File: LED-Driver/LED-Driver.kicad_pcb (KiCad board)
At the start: 2 copper layers, 40.6 x 22.9 mm, 27 parts, among them P1 CONN_02X04, P2 CONN_02X04, P3 CONN_01X05, P4 CONN_01X02, P5 CONN_01X09, P6 CONN_01X09, U1 IS31FL3732

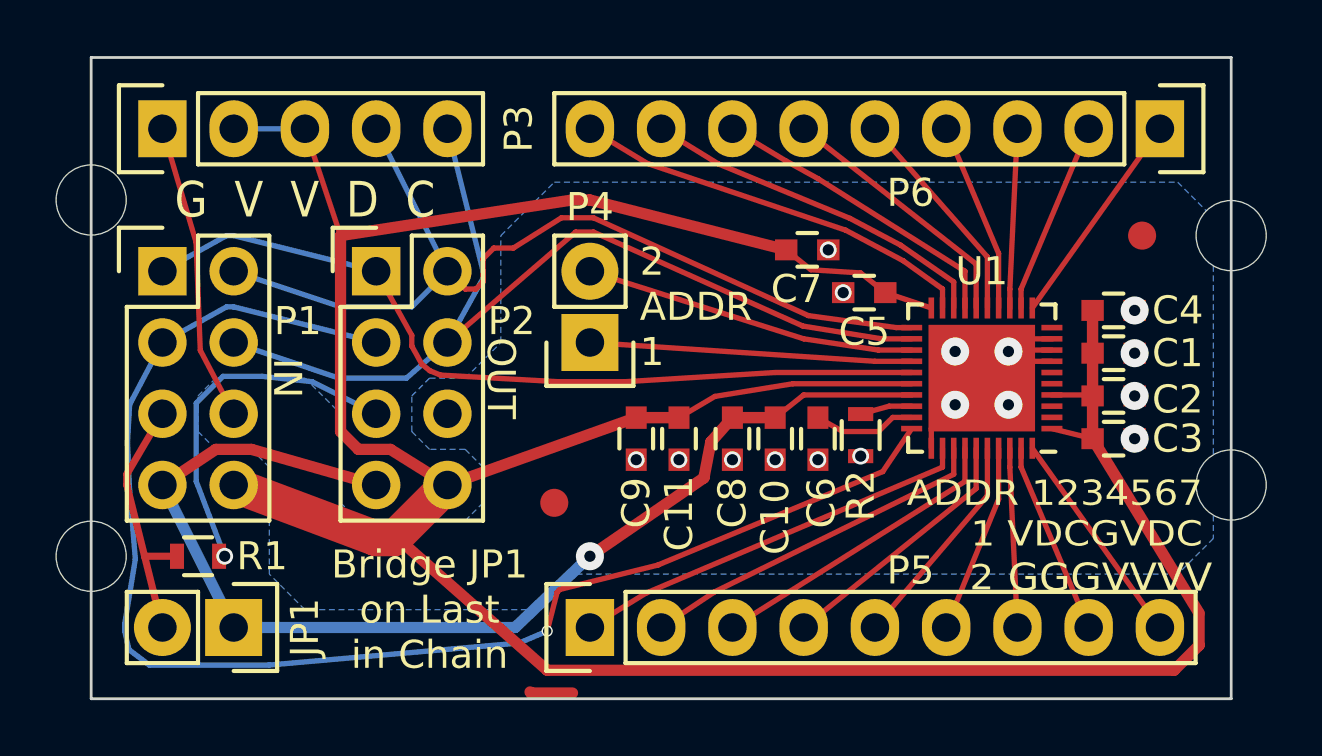
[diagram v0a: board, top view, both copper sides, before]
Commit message: Minor cleanups
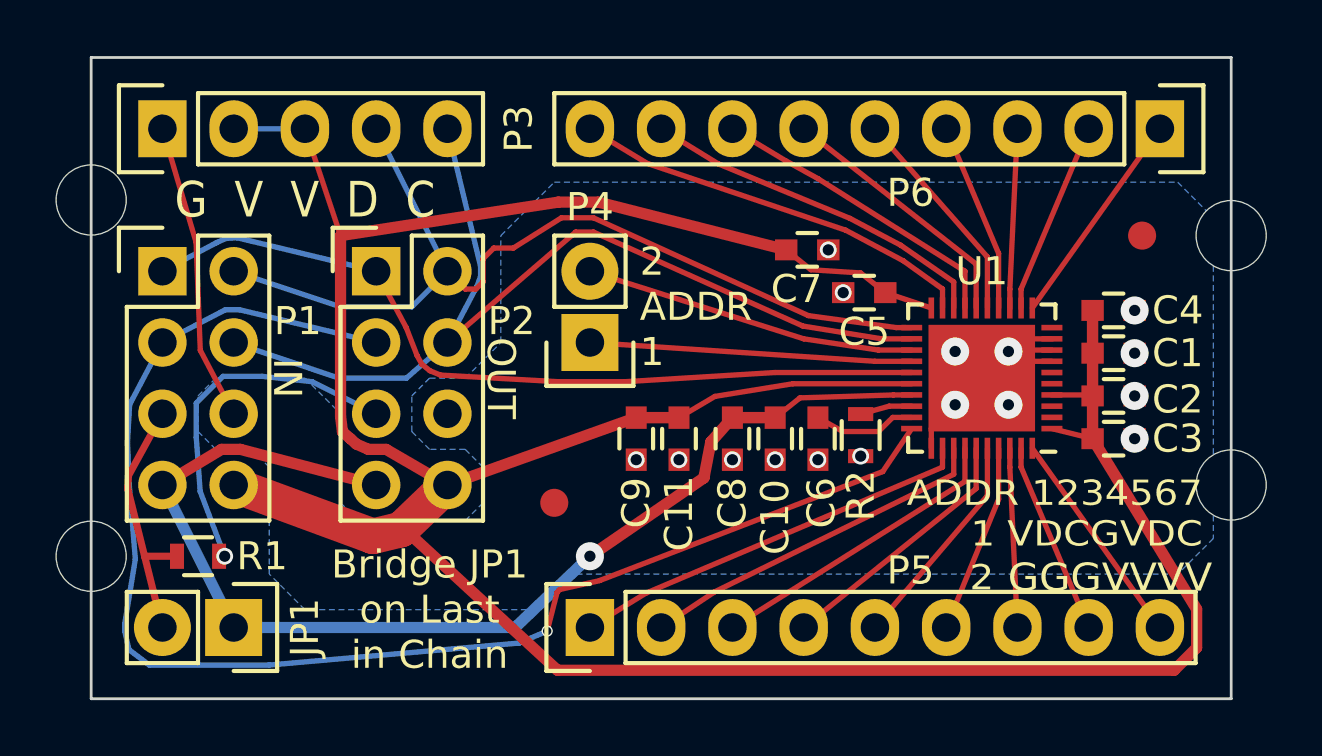
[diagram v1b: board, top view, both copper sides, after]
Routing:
- net (no net): track 1.53 -> 0.00 mm
